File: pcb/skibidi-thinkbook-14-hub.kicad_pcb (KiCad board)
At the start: 4 copper layers, 40 x 70 mm, 121 parts, among them CN1 PJ-325C5-G, U1 HC-USB3.0-C26, U2 TUSB8042AIRGCR, U3 RTL8153B-VB-CG, U4 CH334P, U5 AP63203WU-7, U6 CYA0650-4.7UH, U7 PCM2704CDBR, Y1 24Mhz, Y2 25Mhz, Y3 12Mhz

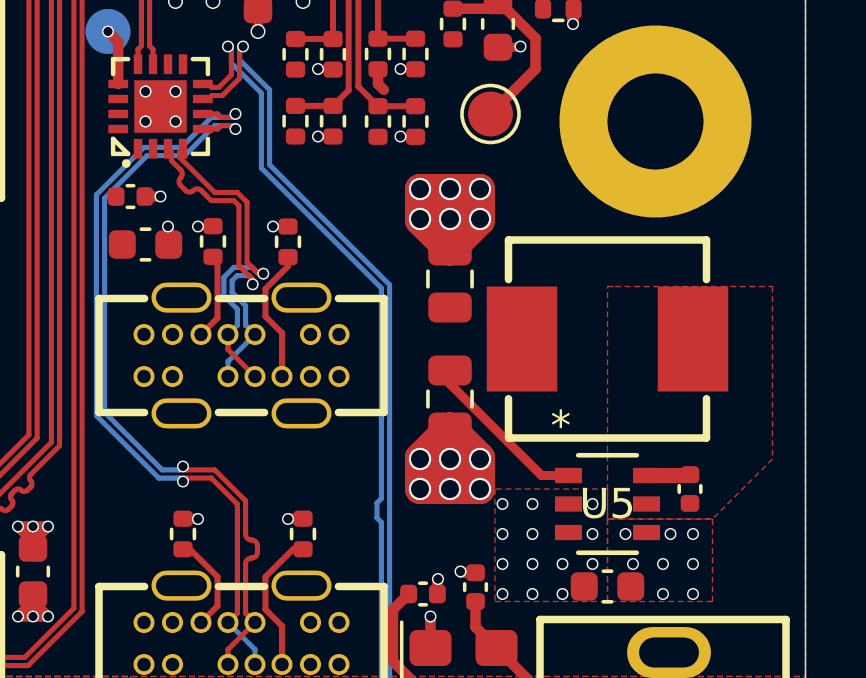
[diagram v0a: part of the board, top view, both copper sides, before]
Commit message: add cad and readme. update pcb a bit too
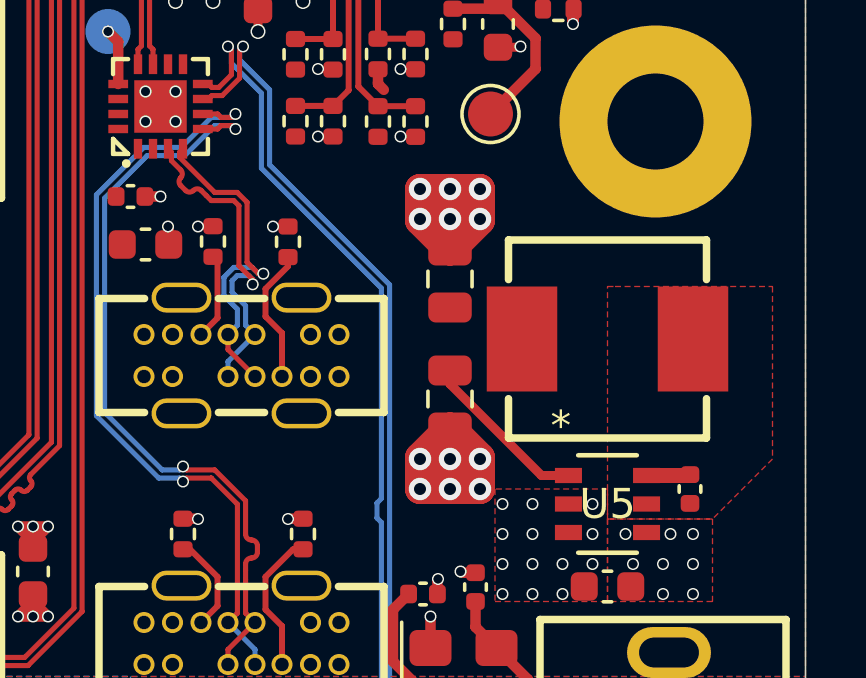
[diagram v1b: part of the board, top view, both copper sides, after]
